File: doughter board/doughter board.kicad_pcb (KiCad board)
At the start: 2 copper layers, 61 x 27.9 mm, 36 parts, among them J1 BOOT_TO/ SELECTOR, J2 BOOT_TO/ SELECTOR, J3 Conn_01x05, J4 RS485, J5 UART2, SW1 SW_SPST, U1 LM1117-3.3, U2 SN65HVD11, U3 STM32F030C6Tx, Y1 8 MHz

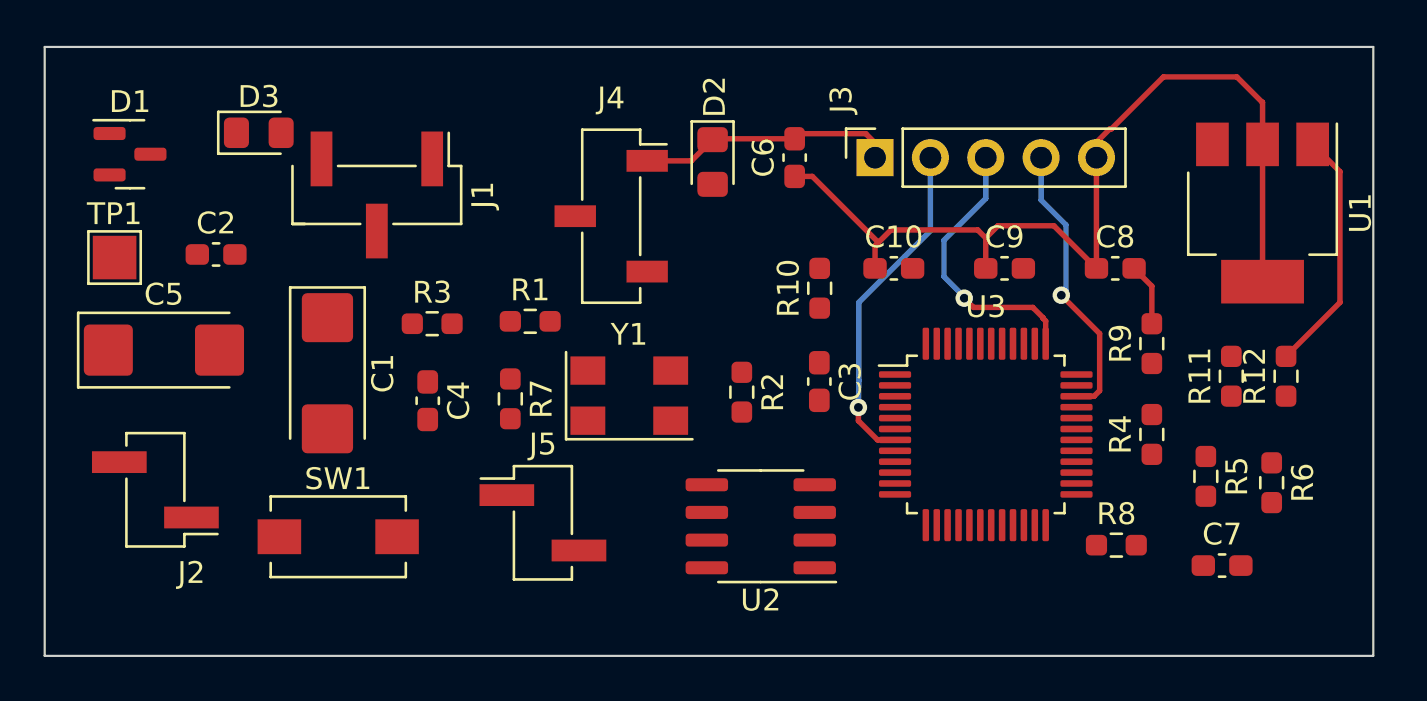
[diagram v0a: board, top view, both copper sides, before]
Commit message: PCB doughter - layout
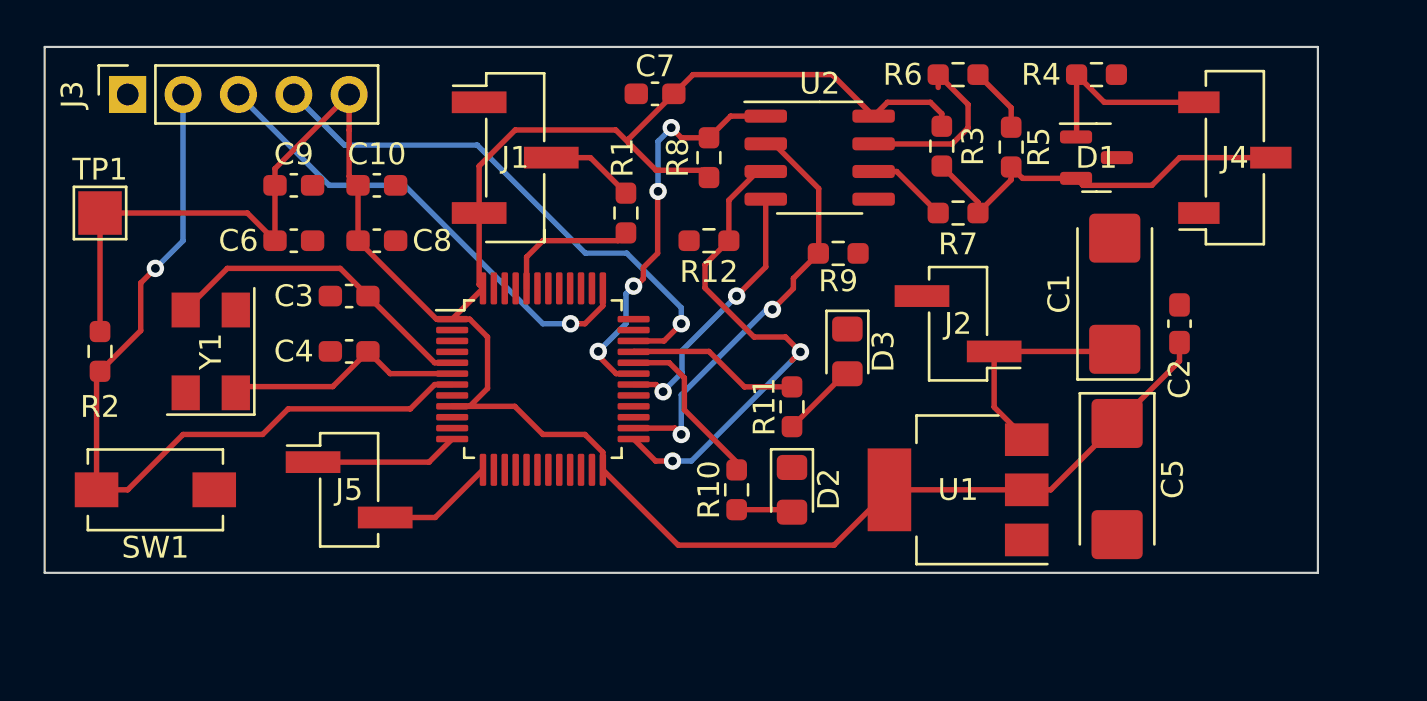
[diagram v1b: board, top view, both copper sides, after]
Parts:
- moved D1 44.3 mm to (157.5, 58.4)
- moved C2 44.3 mm to (161.3, 66.0), turned to 90 degrees
- moved C5 44.1 mm to (158.4, 73.2), turned to -90 degrees
- moved J2 37.6 mm to (151.1, 66.0)
- moved C1 36.3 mm to (158.3, 64.7), turned to 90 degrees
- moved J3 34.4 mm to (113.0, 55.5)
- moved C8 33.9 mm to (124.5, 62.2)
- moved C7 33.8 mm to (137.2, 55.5), turned to 180 degrees
- moved C9 32.8 mm to (120.7, 59.7)
- moved R2 29.5 mm to (111.8, 67.3)
- moved D3 28.8 mm to (146.1, 67.3), turned to -90 degrees
- moved J4 28.7 mm to (163.8, 58.4), turned to 180 degrees
- moved R12 27.2 mm to (139.7, 62.2), turned to 180 degrees
- moved R8 25.8 mm to (139.7, 58.4), turned to 90 degrees
- moved R3 24.8 mm to (150.4, 57.9), turned to -90 degrees
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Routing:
- net +3.3V: track 42.5 -> 120.1 mm
- net GND: track 26.0 -> 1.43 mm
- net DE: track 0.00 -> 23.1 mm, vias 0 -> 2
- net RST: track 15.6 -> 38.1 mm
- net ~{RE}: track 0.00 -> 19.6 mm, vias 0 -> 2
- net UART1_RX_R: track 0.00 -> 19.1 mm, vias 0 -> 4
- net /A: track 0.00 -> 18.4 mm
- net Xtal_IN: track 0.00 -> 14.8 mm
- net UART1_TX_D: track 0.00 -> 12.4 mm, vias 0 -> 2
- net /B: track 0.00 -> 12.1 mm
- net SWD_O: track 13.2 -> 25.1 mm
- net Xtal_OUT: track 0.00 -> 11.1 mm
- net +5V: track 0.00 -> 10.2 mm
- net SWD_CLK: track 12.9 -> 22.2 mm
- net Net-(U2-B): track 0.00 -> 8.62 mm
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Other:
- board size 61 x 27.9 mm -> 58.4 x 24.1 mm
